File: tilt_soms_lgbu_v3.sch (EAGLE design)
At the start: 38 parts, among them Q1 CMG3415

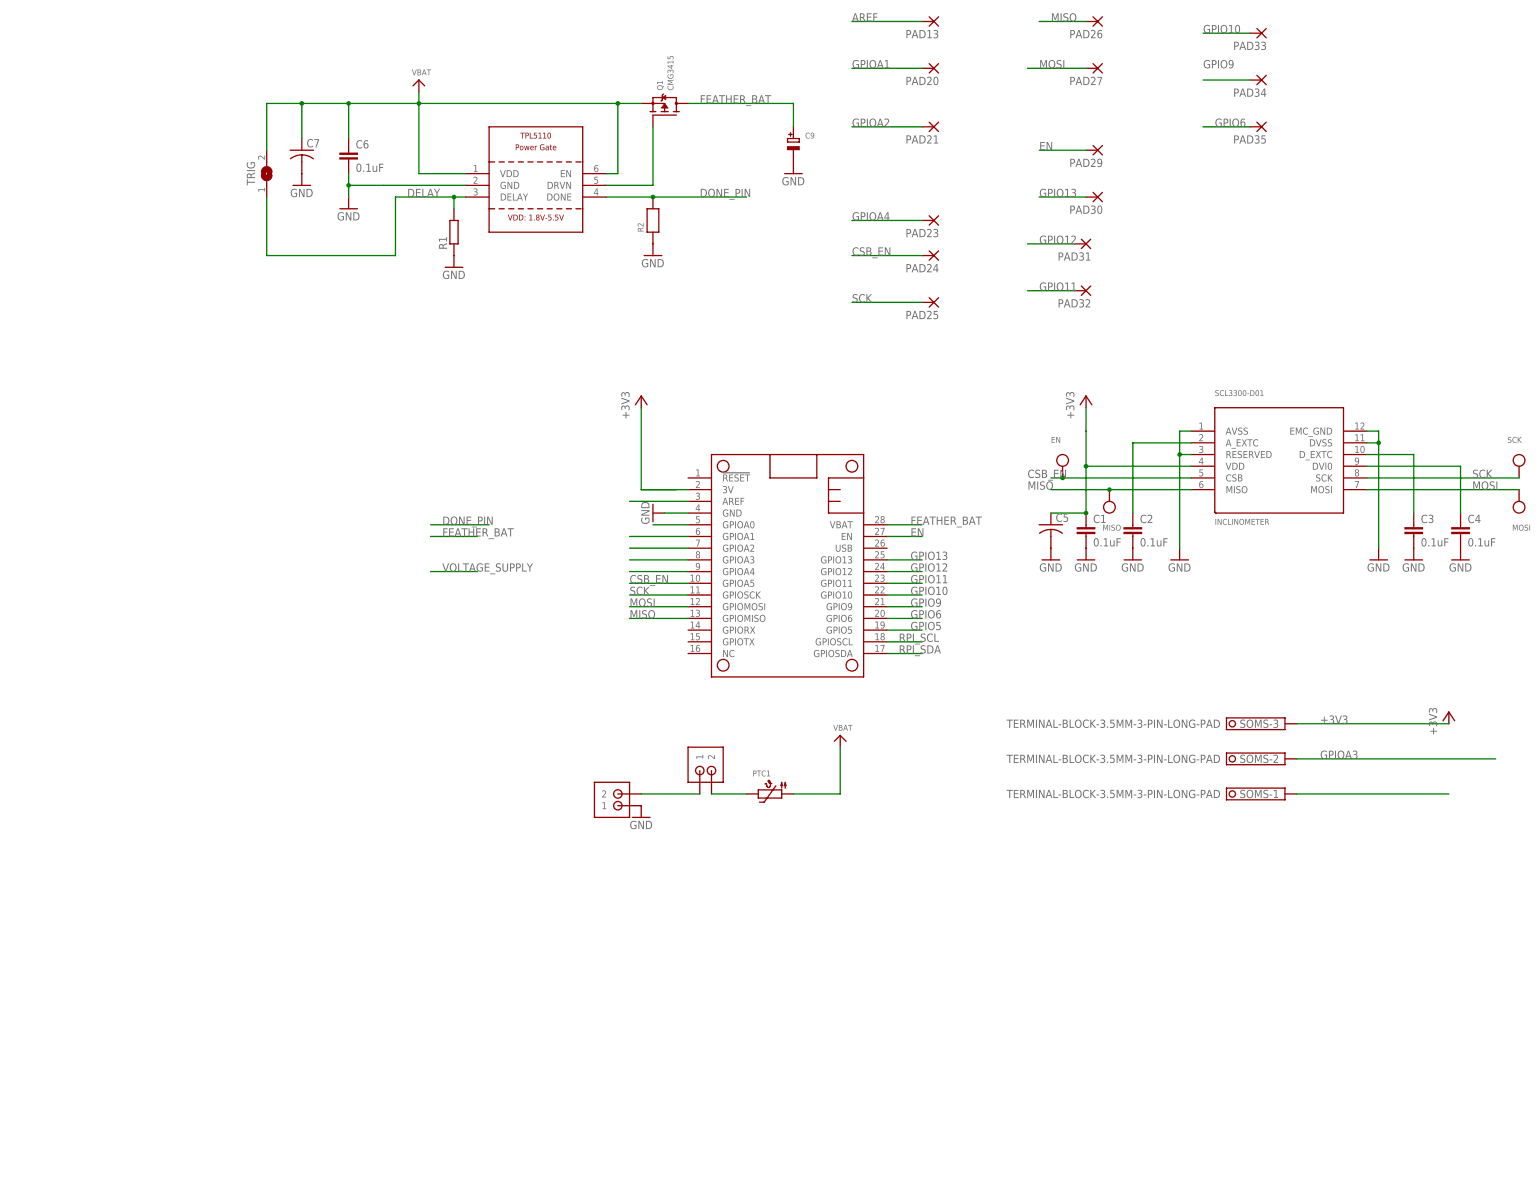
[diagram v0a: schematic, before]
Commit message: ferrite bead, pull ups, standard battery header
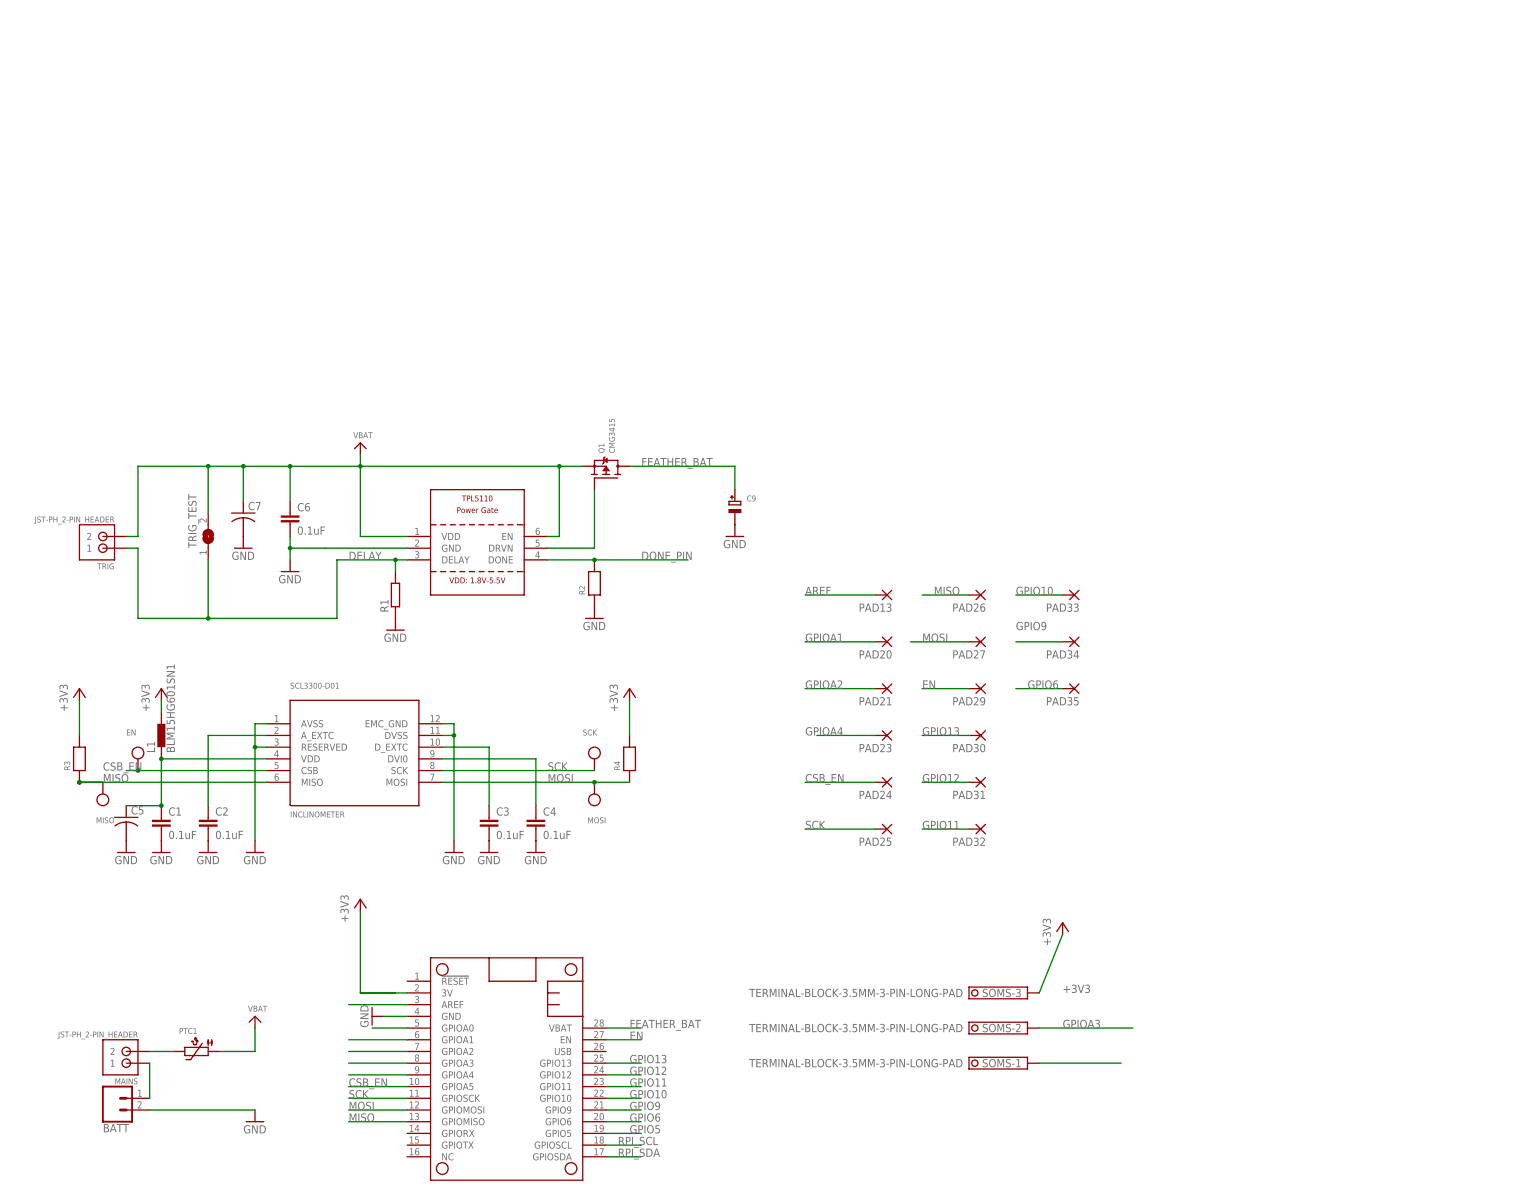
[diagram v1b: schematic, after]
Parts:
- removed MAIN_SWITCH: JST-PH_2-PIN_HEADER, SRG:JST-PH_2-PIN_HEADER
- added L1: BLM15HG601SN1, inductors:BLM15HG601SN1
- added MAINS: JST-PH_2-PIN_HEADER, SRG:JST-PH_2-PIN_HEADER
- added R3, R4: (no value), microbuilder:RESISTOR0805
- added TRIG_TEST: (no value), microbuilder:SOLDERJUMPER
- BATT: value JST-PH_2-PIN_HEADER -> (none); device SRG:JST-PH_2-PIN_HEADER -> SparkFun-Connectors:CONN_02POLAR_LOCK
- R1: device rcl:R-EU_0207/7 -> rcl:R-EU_0207/10
- TRIG: value (none) -> JST-PH_2-PIN_HEADER; device microbuilder:SOLDERJUMPER -> SRG:JST-PH_2-PIN_HEADER
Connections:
- new net N$7: C1.1, C5.1, INCLINOMETER.VDD, L1.1
- net +3V3: now also L1.2, R3.2, R4.2; no longer C1.1, C5.1, INCLINOMETER.VDD
- net DELAY: now also TRIG_TEST.1
- net GND: now also BATT.2; no longer BATT.1
- net MISO: now also R3.1
- net MOSI: now also R4.1
- net N$3: now also BATT.1, MAINS.1; no longer BATT.2, MAIN_SWITCH.1
- net N$4: now also MAINS.2; no longer MAIN_SWITCH.2
- net VBAT: now also TRIG_TEST.2
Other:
- moved on the sheet: C1, C2, C3, C4, C5, C6, C7, C9, EN, INCLINOMETER, MISO, MOSI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
